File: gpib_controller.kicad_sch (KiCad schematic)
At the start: 0 parts

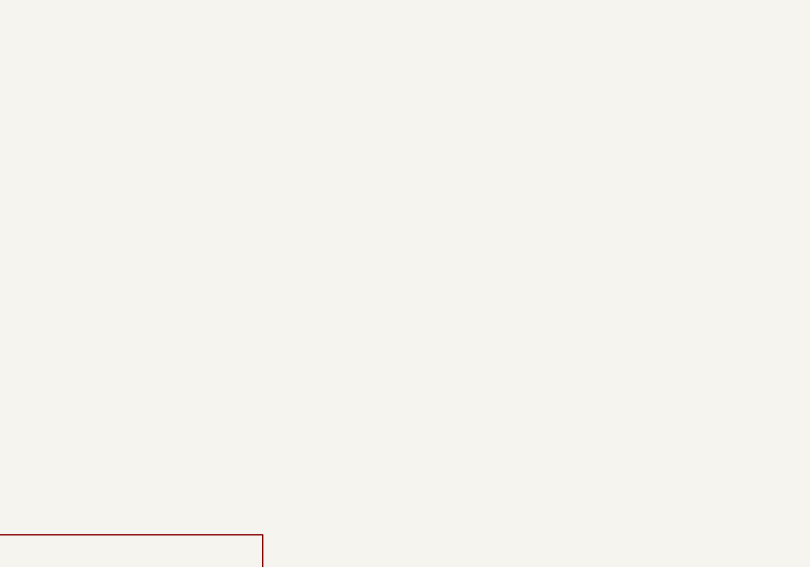
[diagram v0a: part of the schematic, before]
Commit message: Route GPIB pins
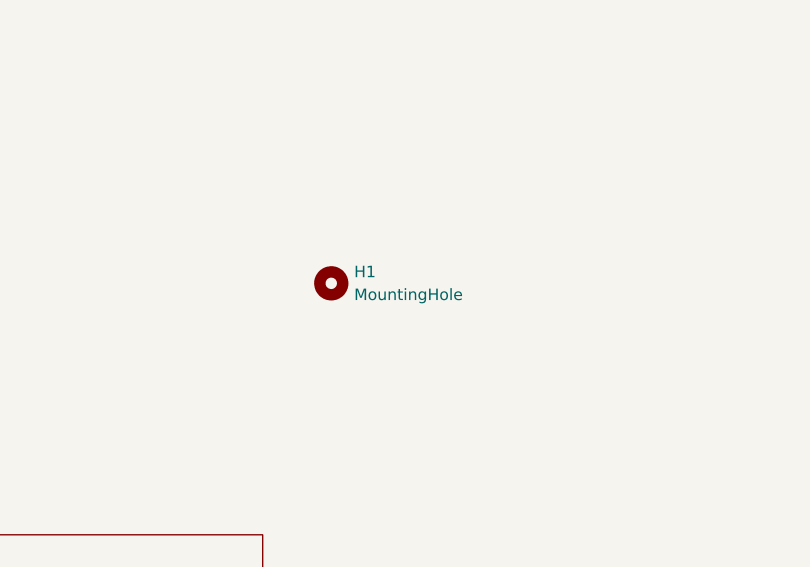
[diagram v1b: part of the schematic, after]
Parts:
- added H1: MountingHole, MountingHole:MountingHole_2.1mm, symbol Mechanical:MountingHole
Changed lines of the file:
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@@
+		)
+	)
+	(symbol
+		(lib_id "Mechanical:MountingHole")
+		(at 109.22 200.66 0)
+		(unit 1)
+		(body_style 1)
+		(exclude_from_sim no)
+		(in_bom no)
+		(on_board yes)
+		(in_pos_files yes)
+		(dnp no)
+		(fields_autoplaced yes)
+		(property "Reference" "H1"
+			(at 111.76 199.39 0)
+			(show_name no)
+			(do_not_autoplace no)
+			(effects
+				(font
+					(size 1.27 1.27)
+				)
+				(justify left)
+			)
+		)
+		(property "Value" "MountingHole"
+			(at 111.76 201.93 0)
+			(show_name no)
+			(do_not_autoplace no)
+			(effects
+				(font
+					(size 1.27 1.27)
+				)
+				(justify left)
+			)
+		)
+		(property "Footprint" "MountingHole:MountingHole_2.1mm"
+			(at 109.22 200.66 0)
+			(hide yes)
+			(show_name no)
+			(do_not_autoplace no)
+			(effects
+				(font
+					(size 1.27 1.27)
+				)
+			)
+		)
+		(property "Datasheet" ""
+			(at 109.22 200.66 0)
+			(hide yes)
+			(show_name no)
+			(do_not_autoplace no)
+			(effects
+				(font
+					(size 1.27 1.27)
+				)
+			)
+		)
+		(property "Description" "Mounting Hole without connection"
+			(at 109.22 200.66 0)
+			(hide yes)
+			(show_name no)
+			(do_not_autoplace no)
+			(effects
+				(font
+					(size 1.27 1.27)
+				)
+			)
+		)
+		(instances
+			(project "gpib_controller"
+				(path "/0f352524-50ff-469d-9a68-783e183b0073"
+					(reference "H1")
+					(unit 1)
+				)
+			)
 		)
 	)
